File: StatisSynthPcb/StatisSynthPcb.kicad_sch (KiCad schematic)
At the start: 21 parts, among them J1 Conn_01x02_Pin, J2 PCM5102A, J3 Oled, J4 Conn pin for power amplifier, SW1 SW_Push, SW2 SW_Push, SW3 SW_Push, SW4 SW_Push, SW5 SW_SPST, U3 MCP3208

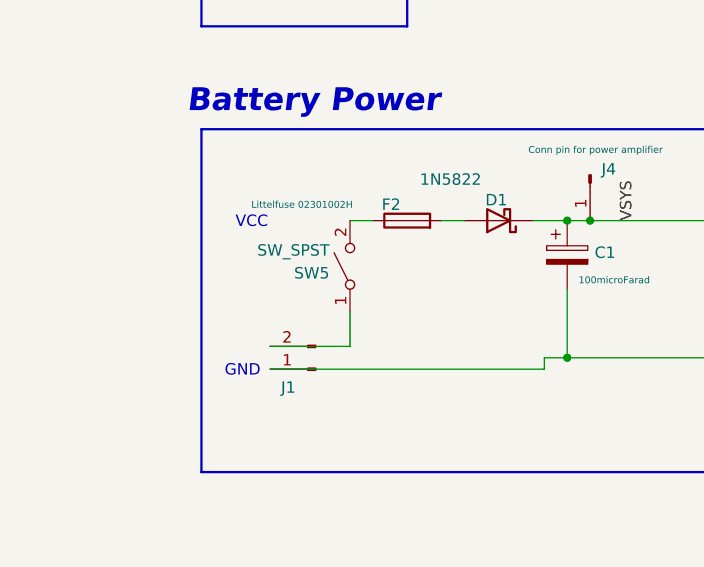
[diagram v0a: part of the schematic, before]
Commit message: added gerbers photos bom
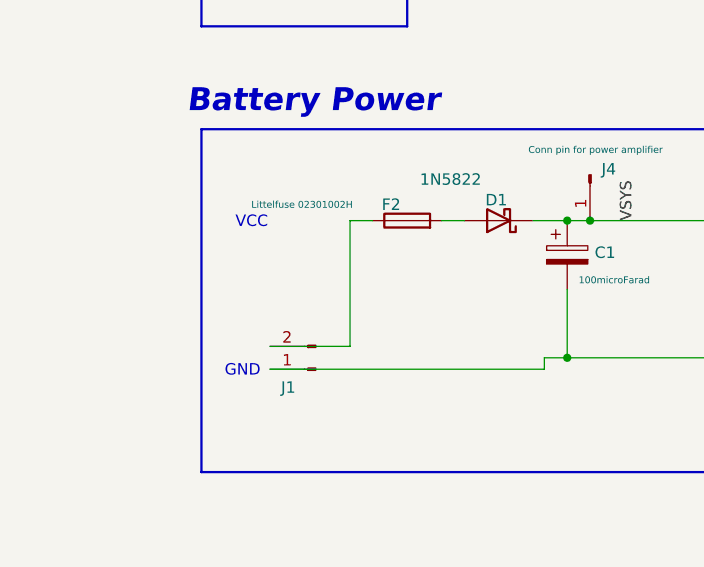
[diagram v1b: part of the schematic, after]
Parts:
- removed SW5: SW_SPST, Button_Switch_THT:SW_DIP_SPSTx01_Slide_9.78x4.72mm_W7.62mm_P2.54mm, symbol Switch:SW_SPST
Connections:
- net at J1.2 (Pin_2): now also F2.1
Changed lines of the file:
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@@
 	(wire
 		(pts
-			(xy 49.53 179.07) (xy 49.53 182.88)
+			(xy 49.53 168.91) (xy 49.53 182.88)
 		)
 		(stroke
@@
 					(unit 1)
 				)
-			)
-		)
-	)
-	(symbol
-		(lib_id "Switch:SW_SPST")
-		(at 49.53 173.99 90)
-		(unit 1)
-		(body_style 1)
-		(exclude_from_sim no)
-		(in_bom yes)
-		(on_board yes)
-		(in_pos_files yes)
-		(dnp no)
-		(property "Reference" "SW5"
-			(at 47.244 174.752 90)
-			(show_name no)
-			(do_not_autoplace no)
-			(effects
-				(font
-					(size 1.27 1.27)
-				)
-				(justify left)
-			)
-		)
-		(property "Value" "SW_SPST"
-			(at 47.244 172.212 90)
-			(show_name no)
-			(do_not_autoplace no)
-			(effects
-				(font
-					(size 1.27 1.27)
-				)
-				(justify left)
-			)
-		)
-		(property "Footprint" "Button_Switch_THT:SW_DIP_SPSTx01_Slide_9.78x4.72mm_W7.62mm_P2.54mm"
-			(at 49.53 173.99 0)
-			(hide yes)
-			(show_name no)
-			(do_not_autoplace no)
-			(effects
-				(font
-					(size 1.27 1.27)
-				)
-			)
-		)
-		(property "Datasheet" ""
-			(at 49.53 173.99 0)
-			(hide yes)
-			(show_name no)
-			(do_not_autoplace no)
-			(effects
-				(font
-					(size 1.27 1.27)
-				)
-			)
-		)
-		(property "Description" "Single Pole Single Throw (SPST) switch"
-			(at 49.53 173.99 0)
-			(hide yes)
-			(show_name no)
-			(do_not_autoplace no)
-			(effects
-				(font
-					(size 1.27 1.27)
-				)
-			)
-		)
-		(pin "1"
-		)
-		(pin "2"
-		)
-		(instances
-			(project "StatisSynthPcb"
-				(path "/b57d530a-5173-4e03-a844-1cb39fed83ec"
-					(reference "SW5")
-					(unit 1)
-				)
